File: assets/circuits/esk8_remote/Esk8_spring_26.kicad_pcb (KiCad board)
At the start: 2 copper layers, 21.9 x 69 mm, 15 parts, among them J1 Conn_01x02_Pin, J2 Conn_01x05_Pin, U8 NRF-MODULE

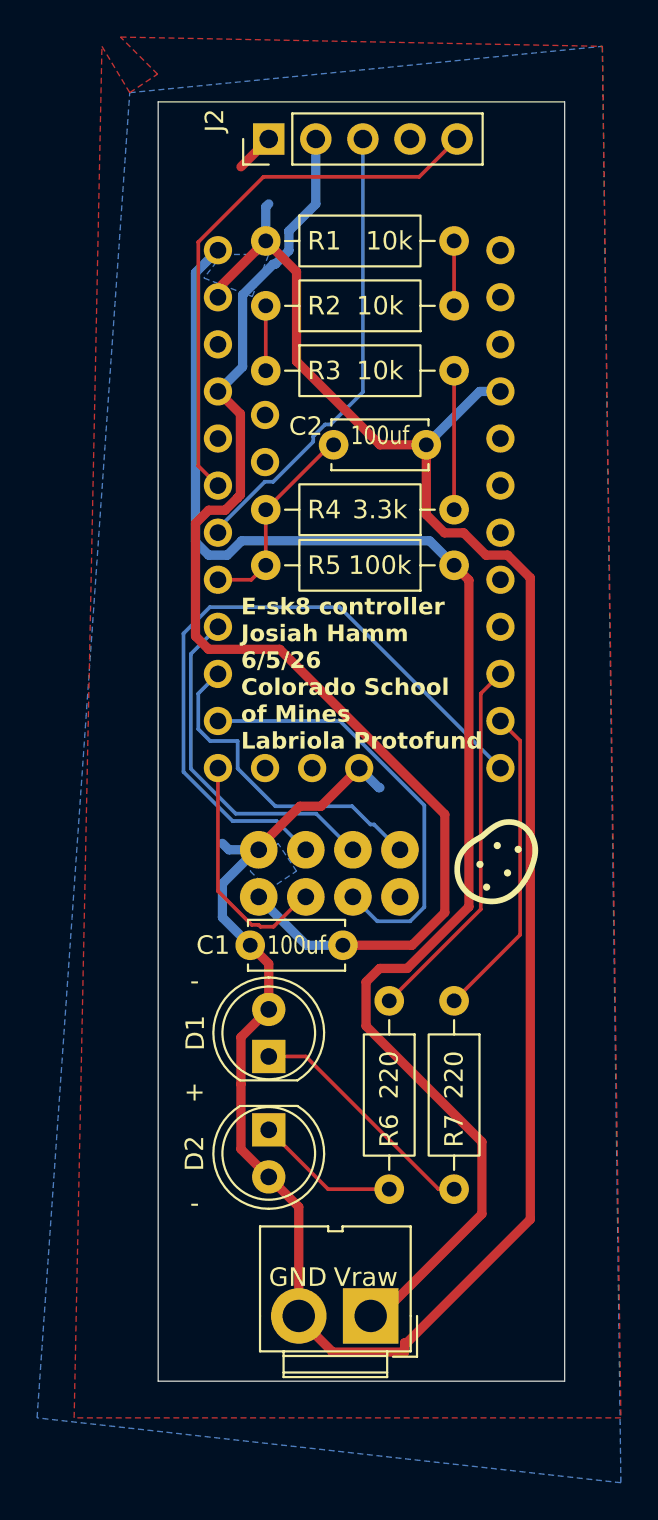
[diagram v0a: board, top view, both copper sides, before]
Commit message: bro I spent 3 hours and changed nothing😭
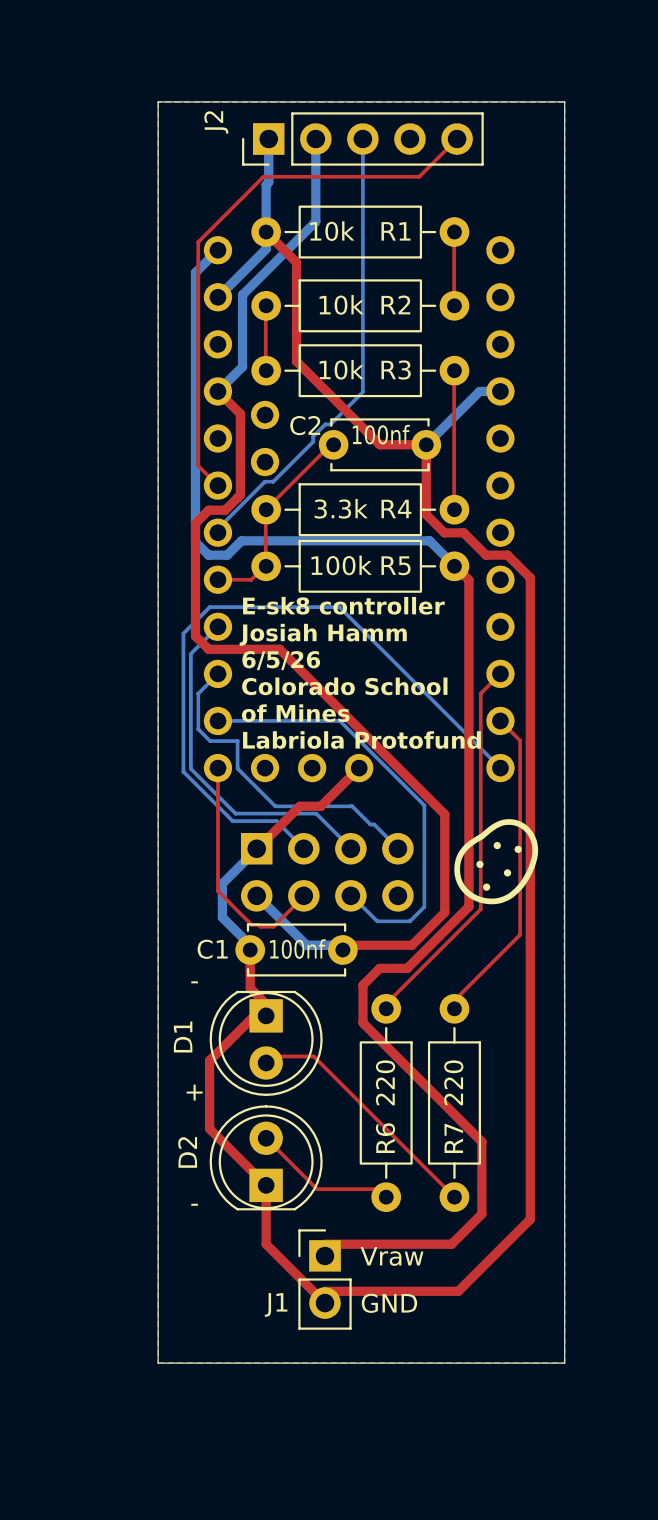
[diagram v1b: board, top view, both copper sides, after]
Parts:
- removed U8: NRF-MODULE, NRF24L01:NRF24Lo1
- added U1: NRF24L01_Breakout, RF_Module:nRF24L01_Breakout, B.Cu at (149.4, 129.8)
- C1, C2: value 100uf -> 100nf
- J1: footprint Connector:JWT_A3963_1x02_P3.96mm_Vertical -> Connector_PinHeader_2.54mm:PinHeader_1x02_P2.54mm_Vertical
- moved R1 10.2 mm to (160.0, 96.5), turned to 180 degrees
- moved R3 10.2 mm to (160.0, 104.0), turned to 180 degrees
- moved R5 10.1 mm to (149.9, 114.6), turned to 0 degrees
- moved R2 10.1 mm to (149.9, 100.5), turned to 0 degrees
- moved R4 10.1 mm to (149.9, 111.5), turned to 0 degrees
- moved J1 4.07 mm to (153.0, 151.8), turned to 0 degrees
- moved D2 3.00 mm to (149.9, 148.0), turned to 90 degrees
- moved D1 2.19 mm to (149.9, 138.8), turned to -90 degrees
- moved R6 0.46 mm to (156.3, 138.4)
- moved R7 0.43 mm to (160.0, 138.4)
- moved C1 0.25 mm to (154.0, 135.3)
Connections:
- net Net-(#U$6-SW) renamed /SW
- net Net-(#U$6-VRX) renamed /VRX
- B2 pad 12: Net-(B2-*9) -> /CE
- B2 pad 13: Net-(B2-*10) -> /CSN
- B2 pad 14: Net-(B2-*11) -> /MOSI
- B2 pad 15: Net-(B2-12) -> /MISO
- B2 pad 16: Net-(B2-13) -> /SCK
- B2 pad 17: Net-(B2-A0) -> /VDIV
- C2 pad 1: Net-(B2-A0) -> /VDIV
- D1 pad 1: Net-(D1-A) -> GND
- D1 pad 2: GND -> Net-(D1-A)
- D2 pad 1: Net-(D2-A) -> GND
- D2 pad 2: GND -> Net-(D2-A)
- R1 pad 1: GND -> Net-(R1-Pad1)
- R1 pad 2: Net-(R1-Pad2) -> GND
- R2 pad 1: Net-(R1-Pad2) -> Net-(R2-Pad1)
- R2 pad 2: Net-(R2-Pad2) -> Net-(R1-Pad1)
- R3 pad 1: Net-(R2-Pad2) -> Net-(R3-Pad1)
- R3 pad 2: Net-(R3-Pad2) -> Net-(R2-Pad1)
- R4 pad 1: Net-(R3-Pad2) -> /VDIV
- R4 pad 2: Net-(B2-A0) -> Net-(R3-Pad1)
- R5 pad 1: Net-(B2-RAW) -> /VDIV
- R5 pad 2: Net-(B2-A0) -> Net-(B2-RAW)
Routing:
- net Net-(B2-*9): track 37.0 -> 0.00 mm
- net /CE: track 0.00 -> 37.0 mm
- net Net-(B2-*11): track 23.2 -> 0.00 mm
- net /MOSI: track 0.00 -> 23.2 mm
- net Net-(B2-13): track 18.7 -> 0.00 mm
- net /SCK: track 0.00 -> 18.7 mm
- net Net-(B2-12): track 17.8 -> 0.00 mm
- net /MISO: track 0.00 -> 17.8 mm
- net Net-(B2-*10): track 12.8 -> 0.00 mm
- net /CSN: track 0.00 -> 12.8 mm
- net Net-(B2-A0): track 11.0 -> 0.00 mm
- net /VDIV: track 0.00 -> 11.0 mm
- net Net-(R3-Pad2): track 7.50 -> 0.00 mm
- net Net-(R3-Pad1): track 0.00 -> 7.50 mm
- net GND: track 132.4 -> 128.3 mm
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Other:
- board size 21.9 x 69 mm -> 21.9 x 68 mm
